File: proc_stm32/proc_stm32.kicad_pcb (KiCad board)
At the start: 2 copper layers, 28 x 18.8 mm, 22 parts, among them J1 Moat_Compute_24, Q1 2N7002, Q2 2N7002, Q3 2N7002, Q4 2N7002, U1 MIC5504, U2 STM32L051K8Tx, U3 LTC4311, U4 LTC4311

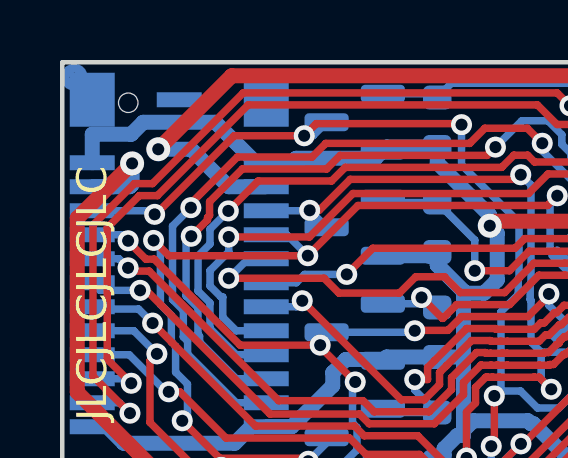
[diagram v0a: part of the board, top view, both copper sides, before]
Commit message: uploads
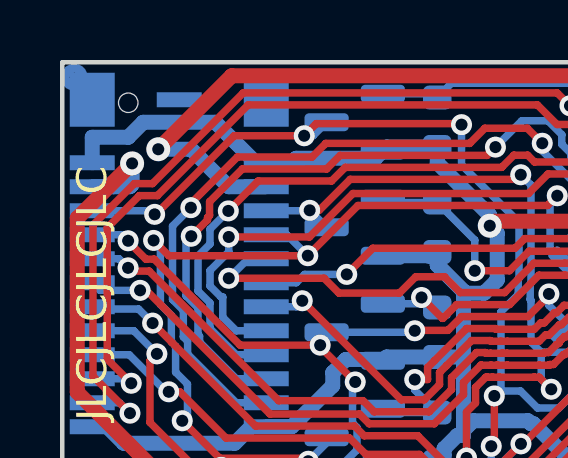
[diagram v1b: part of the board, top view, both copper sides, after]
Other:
- rule pad_to_mask_clearance: 0.051 -> 0
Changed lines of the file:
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@@
 (kicad_pcb (version 20211014) (generator pcbnew)
   (general
-    (thickness 1.6)
+    (thickness 1.09)
   )
   (paper "A4")
@@
   (setup
     (stackup
-      (layer "F.SilkS" (type "Top Silk Screen"))
+      (layer "F.SilkS" (type "Top Silk Screen") (color "White"))
       (layer "F.Paste" (type "Top Solder Paste"))
       (layer "F.Mask" (type "Top Solder Mask") (color "Green") (thickness 0.01))
       (layer "F.Cu" (type "copper") (thickness 0.035))
-      (layer "dielectric 1" (type "core") (thickness 1.51) (material "FR4") (epsilon_r 4.5) (loss_tangent 0.02))
+      (layer "dielectric 1" (type "core") (thickness 1) (material "FR4") (epsilon_r 4.5) (loss_tangent 0.02))
       (layer "B.Cu" (type "copper") (thickness 0.035))
       (layer "B.Mask" (type "Bottom Solder Mask") (color "Green") (thickness 0.01))
       (layer "B.Paste" (type "Bottom Solder Paste"))
-      (layer "B.SilkS" (type "Bottom Silk Screen"))
+      (layer "B.SilkS" (type "Bottom Silk Screen") (color "White"))
       (copper_finish "None")
       (dielectric_constraints no)
     )
-    (pad_to_mask_clearance 0.051)
-    (solder_mask_min_width 0.25)
+    (pad_to_mask_clearance 0)
     (grid_origin 145 137.2)
     (pcbplotparams
@@
   (segment (start 49.999501 51.760455) (end 49.560455 52.199501) (width 0.5) (layer "B.Cu") (net 1))
   (segment (start 44.516334 54.846487) (end 44.95538 54.407441) (width 0.5) (layer "B.Cu") (net 1))
+  (segment (start 36.5 47.85) (end 36.5 47) (width 0.5) (layer "B.Cu") (net 1))
   (segment (start 56.225 45.575) (end 56.225 47.243629) (width 0.5) (layer "B.Cu") (net 1))
   (segment (start 56.800509 48.466476) (end 56.208976 49.058009) (width 0.5) (layer "B.Cu") (net 1))
@@
   (segment (start 52.716492 58.778992) (end 52.716492 58.166492) (width 0.5) (layer "B.Cu") (net 1))
   (segment (start 44.74952 59.38798) (end 46.1875 57.95) (width 0.25) (layer "B.Cu") (net 1))
-  (segment (start 38.2 46.5) (end 40.600978 46.5) (width 0.5) (layer "B.Cu") (net 1))
+  (segment (start 36.5 47) (end 37.7 47) (width 0.5) (layer "B.Cu") (net 1))
   (segment (start 43.35 47.85) (end 42.3 47.85) (width 0.5) (layer "B.Cu") (net 1))
   (segment (start 55.2625 60.1) (end 54.65 60.7125) (width 0.5) (layer "B.Cu") (net 1))
@@
   (segment (start 44 62.275) (end 44.74952 61.52548) (width 0.25) (layer "B.Cu") (net 1))
   (segment (start 51.124062 56.549011) (end 51.02555 56.450499) (width 0.5) (layer "B.Cu") (net 1))
-  (segment (start 36.5 47.85) (end 36.5 46.900511) (width 0.5) (layer "B.Cu") (net 1))
   (segment (start 57.4 58.050001) (end 58.255888 57.194113) (width 0.5) (layer "B.Cu") (net 1))
   (segment (start 42.024511 62.724511) (end 43.550489 62.724511) (width 0.25) (layer "B.Cu") (net 1))
@@
   (segment (start 52.525 57.865044) (end 51.208968 56.549012) (width 0.5) (layer "B.Cu") (net 1))
   (segment (start 46.3125 57.825) (end 46.1875 57.95) (width 0.5) (layer "B.Cu") (net 1))
+  (segment (start 40.600978 46.5) (end 41.950978 47.85) (width 0.5) (layer "B.Cu") (net 1))
   (segment (start 62.301821 48.751821) (end 62.75 49.2) (width 0.5) (layer "B.Cu") (net 1))
   (segment (start 49.198541 56.450499) (end 48.87452 56.77452) (width 0.5) (layer "B.Cu") (net 1))
@@
   (segment (start 49.999501 50.199501) (end 49.75 49.95) (width 0.5) (layer "B.Cu") (net 1))
   (segment (start 46 62.7) (end 45.675499 63.024501) (width 0.25) (layer "B.Cu") (net 1))
-  (segment (start 36.5 46.900511) (end 37.799489 46.900511) (width 0.5) (layer "B.Cu") (net 1))
-  (segment (start 37.799489 46.900511) (end 38.2 46.5) (width 0.5) (layer "B.Cu") (net 1))
   (segment (start 45.57629 54.407441) (end 45.618849 54.45) (width 0.5) (layer "B.Cu") (net 1))
   (segment (start 46.1875 50.95) (end 47.875 50.95) (width 0.5) (layer "B.Cu") (net 1))
@@
   (segment (start 57.65 60.1) (end 55.2625 60.1) (width 0.5) (layer "B.Cu") (net 1))
   (segment (start 49.999501 51.760455) (end 49.999501 50.199501) (width 0.5) (layer "B.Cu") (net 1))
-  (segment (start 40.600978 46.5) (end 41.950978 47.85) (width 0.5) (layer "B.Cu") (net 1))
   (segment (start 48 51.009956) (end 48 50.825) (width 0.5) (layer "B.Cu") (net 1))
   (segment (start 54.65 60.7125) (end 52.716492 58.778992) (width 0.5) (layer "B.Cu") (net 1))
@@
   (segment (start 56.225 47.243629) (end 56.311344 47.329973) (width 0.5) (layer "B.Cu") (net 1))
   (segment (start 42.3 56.65) (end 43.147862 56.65) (width 0.5) (layer "B.Cu") (net 1))
-  (segment (start 41.950978 47.85) (end 42.3 47.85) (width 0.5) (layer "B.Cu") (net 1))
   (segment (start 37.55 57.2) (end 41.25 57.2) (width 0.5) (layer "B.Cu") (net 1))
   (segment (start 37 56.65) (end 37.55 57.2) (width 0.5) (layer "B.Cu") (net 1))
   (segment (start 41.25 57.2) (end 41.8 56.65) (width 0.5) (layer "B.Cu") (net 1))
+  (segment (start 37.7 47) (end 38.2 46.5) (width 0.5) (layer "B.Cu") (net 1))
+  (segment (start 38.2 46.5) (end 40.600978 46.5) (width 0.5) (layer "B.Cu") (net 1))
   (segment (start 48.87452 56.941882) (end 48.87452 54.32548) (width 0.5) (layer "B.Cu") (net 1))
   (segment (start 46.3125 54.325) (end 48 54.325) (width 0.5) (layer "B.Cu") (net 1))
@@
   (segment (start 44 62.283179) (end 44 62.275) (width 0.25) (layer "B.Cu") (net 1))
   (segment (start 57.4 59.2) (end 57.4 59.85) (width 0.5) (layer "B.Cu") (net 1))
+  (segment (start 41.950978 47.85) (end 42.3 47.85) (width 0.5) (layer "B.Cu") (net 1))
   (segment (start 48.665104 56.941882) (end 48.87452 56.941882) (width 0.5) (layer "B.Cu") (net 1))
   (segment (start 49.901978 57.198022) (end 49.901978 55.622552) (width 0.25) (layer "F.Cu") (net 2))

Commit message: No save for too long …
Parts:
- C4, C5: value 1µ -> 1µF
- C6: value 100n -> 100nF
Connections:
- U1 pad 4: (no net) -> unconnected-(U1-NC)
- U3 pad 5: (no net) -> unconnected-(U3-NC)
- U4 pad 5: (no net) -> unconnected-(U4-NC)
